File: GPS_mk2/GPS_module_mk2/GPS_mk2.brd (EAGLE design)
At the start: 38.1 x 38.1 mm, 15 parts, among them IC1 MAX3232CSE

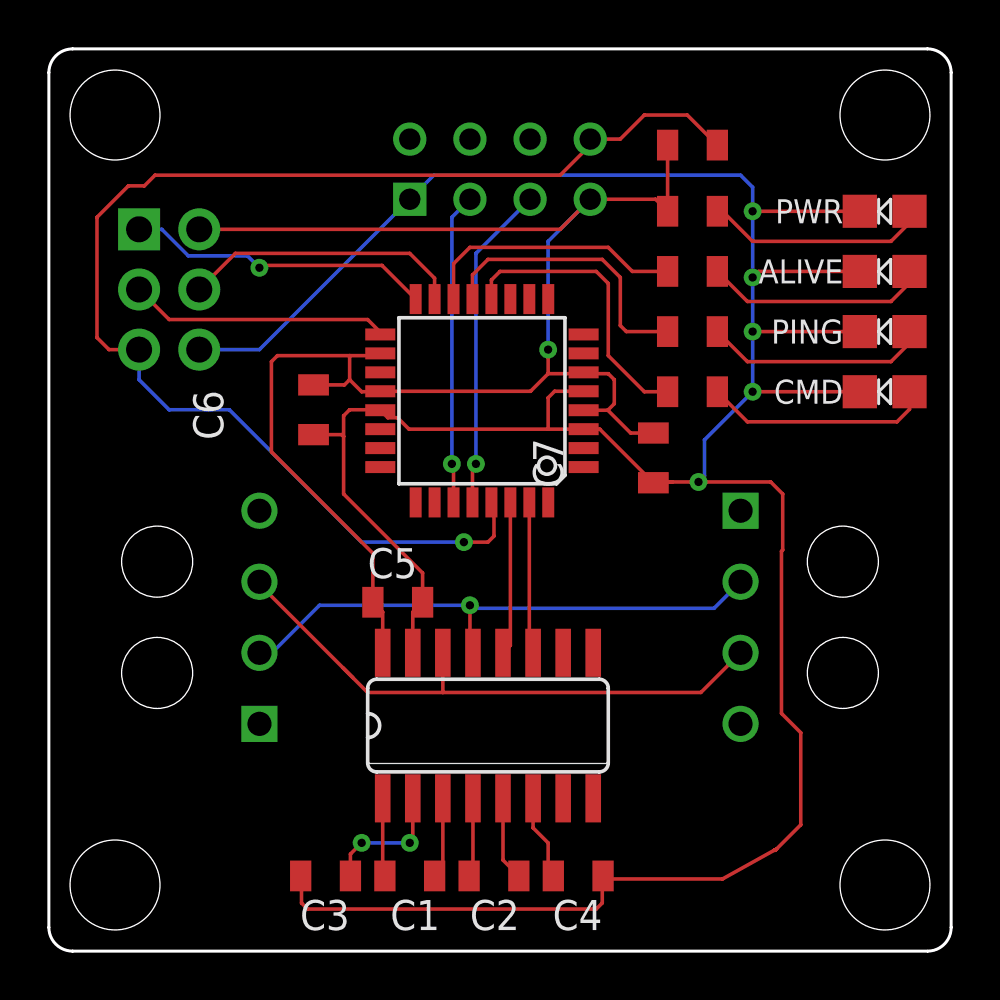
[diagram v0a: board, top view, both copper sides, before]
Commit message: IMU layout. GPS layout tweaks
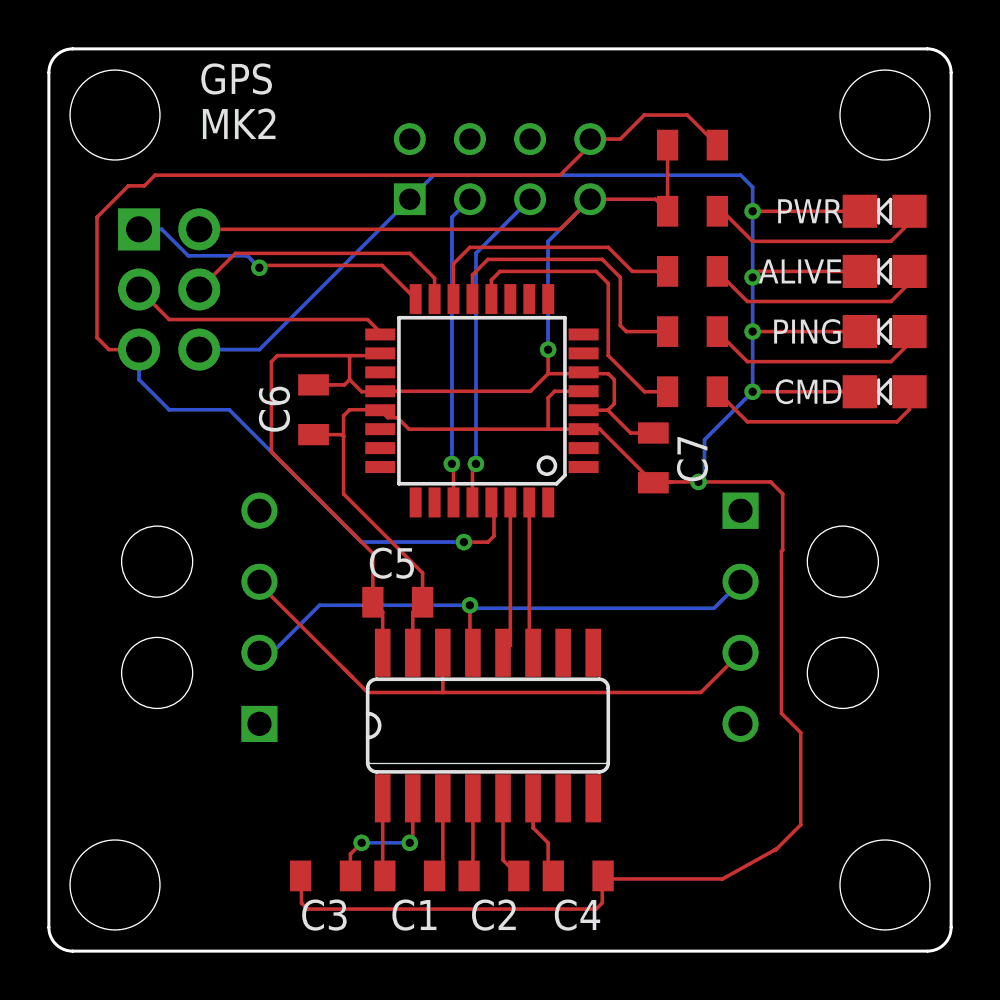
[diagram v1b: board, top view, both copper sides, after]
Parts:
- GPS: value SENSOR_MODULE_MK1 -> MK2
- renumbered GPS_MK2 to GPS
